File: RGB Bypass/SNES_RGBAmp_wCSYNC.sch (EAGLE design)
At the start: 31 parts, among them J3 SNES_MULTIAV_RGBC_ONLY, U1 THS7374

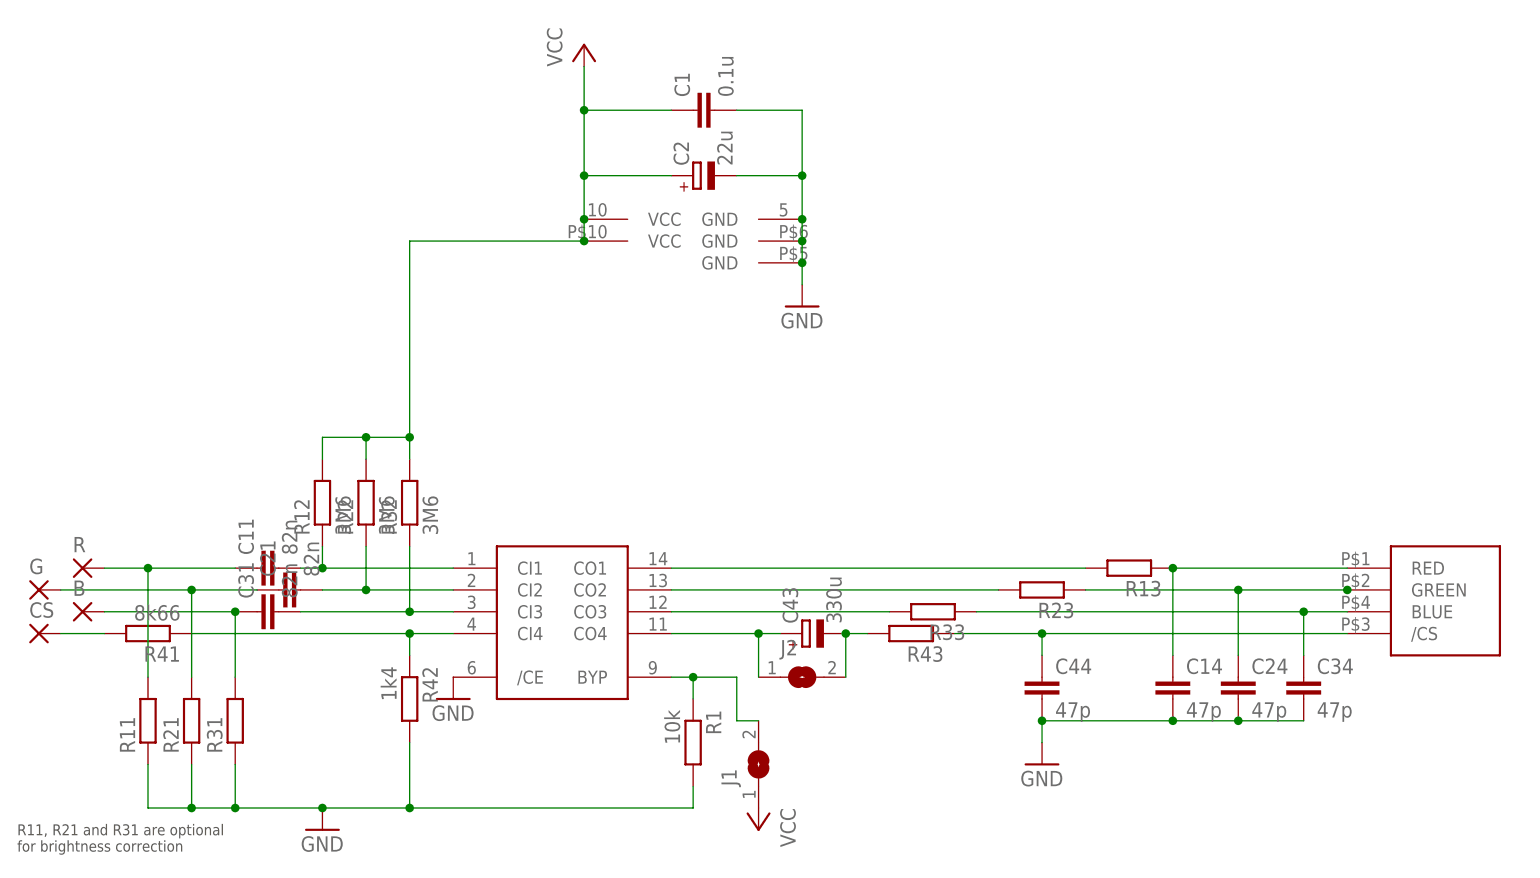
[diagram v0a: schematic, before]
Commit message: go to version 4.1
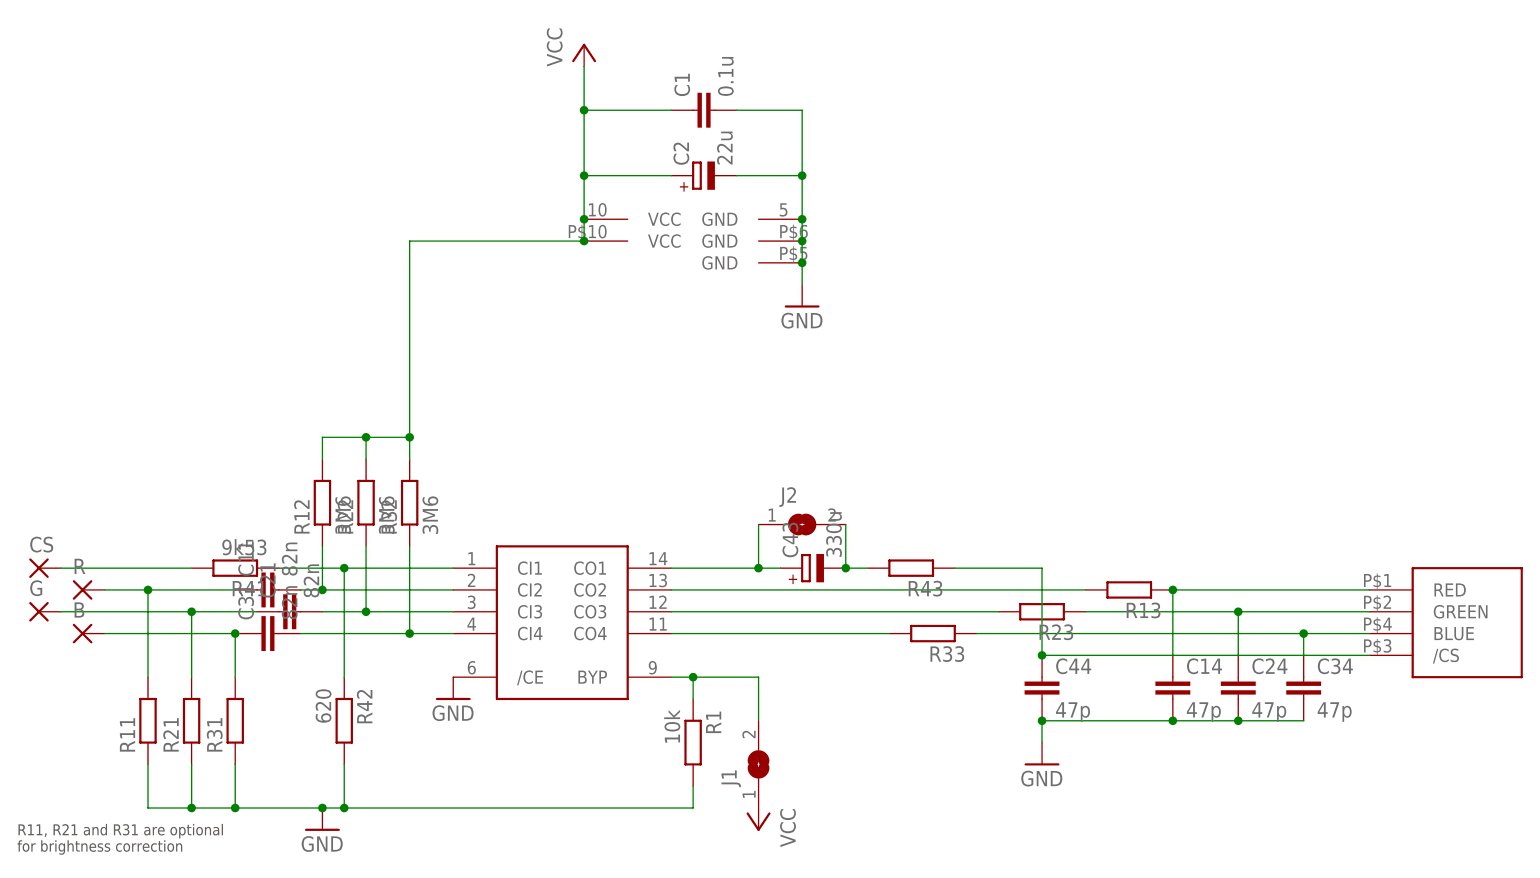
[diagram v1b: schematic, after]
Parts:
- R41: value 8k66 -> 9k53
- R42: value 1k4 -> 620
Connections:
- removed net N$12: R13.2, U1G$1.CO1
- removed net N$13: R23.2, U1G$1.CO2
- new net N$11: R33.2, U1G$1.CO4
- new net N$7: R23.2, U1G$1.CO3
- net N$1: now also U1G$1.CI2; no longer U1G$1.CI1
- net N$10: now also U1G$1.CI1; no longer U1G$1.CI4
- net N$18: now also U1G$1.CO1; no longer U1G$1.CO4
- net N$2: now also U1G$1.CI3; no longer U1G$1.CI2
- net N$8: now also R13.2, U1G$1.CO2; no longer R33.2, U1G$1.CO3
- net R9: now also U1G$1.CI4; no longer U1G$1.CI3
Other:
- moved on the sheet: B, C11, C21, C31, C43, CS, G, J2, R, R13, R23, R33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
